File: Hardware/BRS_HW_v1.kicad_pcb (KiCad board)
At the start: 2 copper layers, 52.6 x 88.8 mm, 128 parts, among them J1 BATTERY, J2 USB_C_Receptacle_USB2.0_14P, J3 SWD/ExtTrig, J4 EXT_GPIOS, J5 Micro_SD_Card, J6 RCV_SYS, J7 RBF_SYS, J8 GND, J9 3V3, Q1 PMOS, Q2 PMOS, Q3 AO3401A, Q4 AO3401A, Q5 BC848, Q6 BC848, Q7 BC848, Q8 AO3400A, SW1 ON/OFF MECH, SW2 SW_MCU_NRST, U1 AMS1117-3.3, U2 USBLC6-2, U3 STM32F411CEUx, U4 CAT811TTBI-GT3, U5 W25Q128JVS, U6 MPU-6000, U7 BMP280, U8 TCA9534, Y1 16MHz

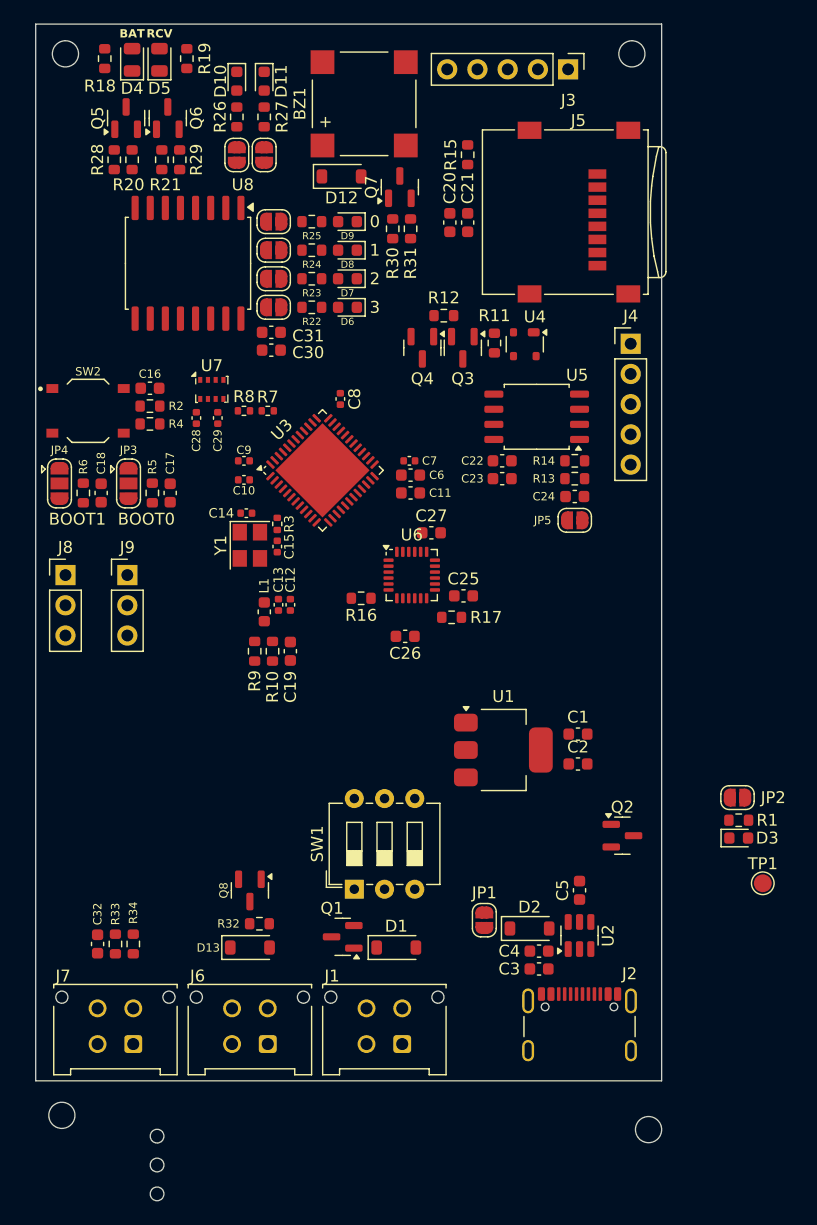
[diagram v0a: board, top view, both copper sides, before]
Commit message: Developing HW - routing
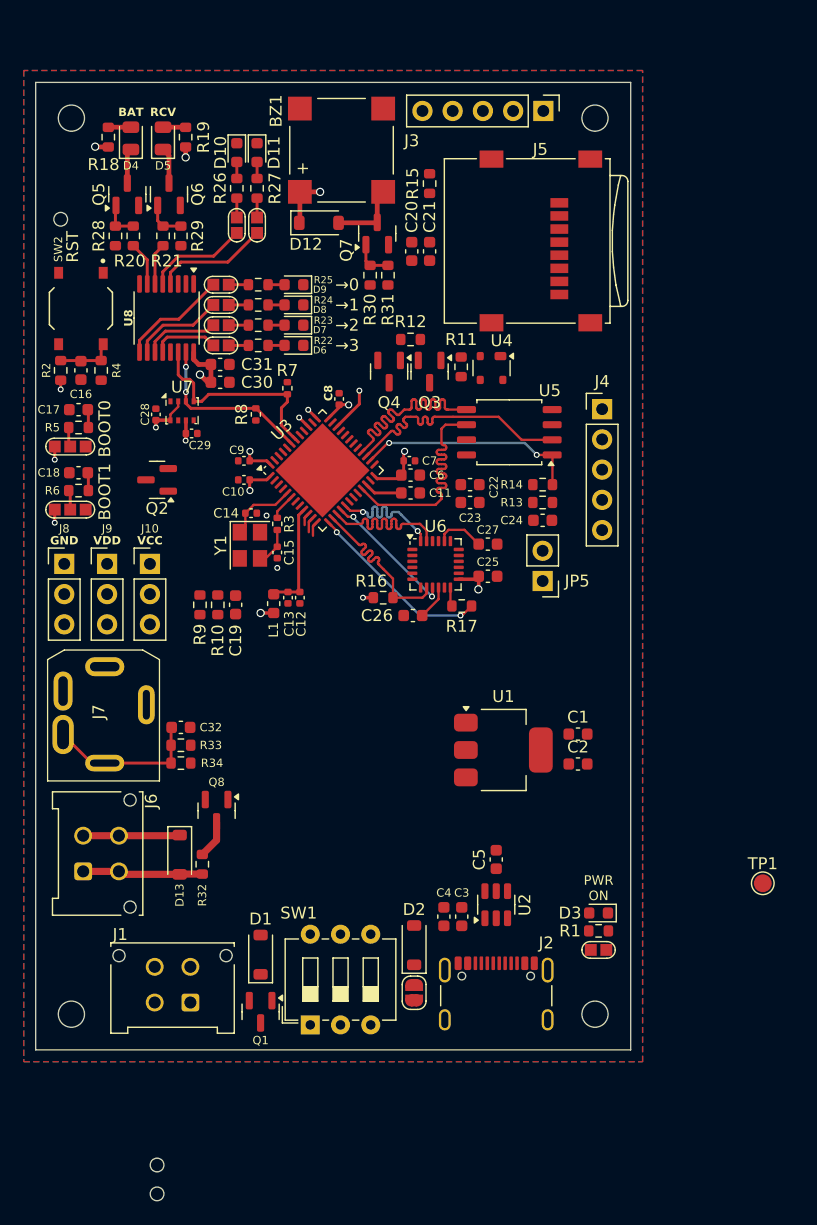
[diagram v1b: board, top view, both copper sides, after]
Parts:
- added J10: VCC, Connector_PinHeader_2.54mm:PinHeader_1x03_P2.54mm_Vertical, F.Cu at (107.1, 117.9)
- J7: footprint Connector_Molex:Molex_Micro-Fit_3.0_43045-0412_2x02_P3.00mm_Vertical -> BRS_Footprints:AudioJack_Vertical
- J9: value 3V3 -> VDD
- JP10, JP11, JP2, JP6, JP7, JP8, JP9: footprint Jumper:SolderJumper-2_P1.3mm_Open_RoundedPad1.0x1.5mm -> BRS_Footprints:SMD_SolderJumper_Small
- JP3, JP4: footprint Jumper:SolderJumper-3_P1.3mm_Open_RoundedPad1.0x1.5mm -> BRS_Footprints:SMD_SolderJumper_Triple_Small
- JP5: footprint Jumper:SolderJumper-2_P1.3mm_Open_RoundedPad1.0x1.5mm -> Connector_PinHeader_2.54mm:PinHeader_1x02_P2.54mm_Vertical
- U8: footprint Package_SO:SOIC-16W_7.5x10.3mm_P1.27mm -> Package_SO:TSSOP-16_4.4x5mm_P0.65mm
- moved H2 77.5 mm to (99.6, 88.9)
- moved Q2 49.2 mm to (107.7, 110.8), turned to 180 degrees
- moved J7 28.0 mm to (103.3, 130.3), turned to 90 degrees
- moved J6 21.2 mm to (101.5, 143.7), turned to 90 degrees
- moved C32 19.5 mm to (109.7, 131.6), turned to 0 degrees
- moved J1 18.1 mm to (110.5, 154.7)
- moved R33 17.6 mm to (109.7, 133.1), turned to 0 degrees
- moved JP2 17.3 mm to (144.8, 150.3), turned to 180 degrees
- moved R34 15.7 mm to (109.7, 134.6), turned to 180 degrees
- moved R1 15.0 mm to (144.8, 148.7), turned to 180 degrees
- moved D3 13.4 mm to (144.8, 147.2), turned to 180 degrees
- moved SW1 12.0 mm to (120.6, 156.6)
- moved D1 11.4 mm to (116.4, 150.7), turned to 90 degrees
- moved H7 10.7 mm to (144.5, 155.7)
- moved C17 10.4 mm to (101.1, 104.9), turned to 180 degrees
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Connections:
- C32 pad 1: Net-(J7-Pin_1) -> Net-(J7-T)
- J7 pad 1: Net-(J7-Pin_1) -> GND
- J7 pad 2: GND -> Net-(J7-T)
- J7 pad 3: Net-(J7-Pin_1) -> unconnected-(J7-R-Pad3)
- J7 pad 4: GND -> Net-(J7-T)
- R33 pad 1: Net-(J7-Pin_1) -> Net-(J7-T)
- R34 pad 2: Net-(J7-Pin_1) -> Net-(J7-T)
- R9 pad 2: +BATT -> HV_PWR_IN
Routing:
- net SYS_SWDIO: track 0.00 -> 35.0 mm, vias 0 -> 1
- net SYS_SWCLK: track 0.00 -> 33.7 mm, vias 0 -> 1
- net SYS_SWO: track 0.00 -> 32.8 mm, vias 0 -> 1
- net VDD: track 0.00 -> 27.7 mm, vias 0 -> 12
- net SPI2_MISO: track 0.00 -> 21.8 mm
- net SPI2_SCK: track 0.00 -> 21.7 mm
- net SPI2_MOSI: track 0.00 -> 21.7 mm
- net SPI2_NSS0: track 0.00 -> 18.8 mm, vias 0 -> 2
- net I2C_SCL: track 0.00 -> 17.6 mm
- net IMU_INT: track 0.00 -> 15.7 mm, vias 0 -> 2
- net SPI1_NSS: track 0.00 -> 15.0 mm
- net I2C_SDA: track 0.00 -> 14.6 mm, vias 0 -> 2
- net SPI1_SCK: track 0.00 -> 14.5 mm
- net Net-(J7-T): track 0.00 -> 13.1 mm
- net SPI1_MISO: track 0.00 -> 11.5 mm, vias 0 -> 2
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- added copper zone on B.Cu, net GND
- added copper zone on F.Cu, net GND
- added copper zone on In1.Cu, net GND
- added copper zone on In4.Cu, net GND
- added copper zone on In3.Cu, net VCC
- added copper zone on In2.Cu, net VDD
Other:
- board size 52.6 x 88.8 mm -> 50 x 81.3 mm
- copper layers 2 -> 6
- board text added: "GND"
- board text added: "PWR ON"
- board text added: "RST"
- board text added: "VCC"
- board text added: "VDD"
- board text added: "→0"
- board text added: "→1"
- board text added: "→2"
- board text added: "→3"
- board text removed: "0"
- board text removed: "1"
- board text removed: "2"
- board text removed: "3"
